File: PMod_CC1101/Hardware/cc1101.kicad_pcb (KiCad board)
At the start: 4 copper layers, 40.5 x 17 mm, 18 parts, among them J1 Conn_Coaxial, J2 Conn_02x06_Odd_Even, U1 CC1101RGPR

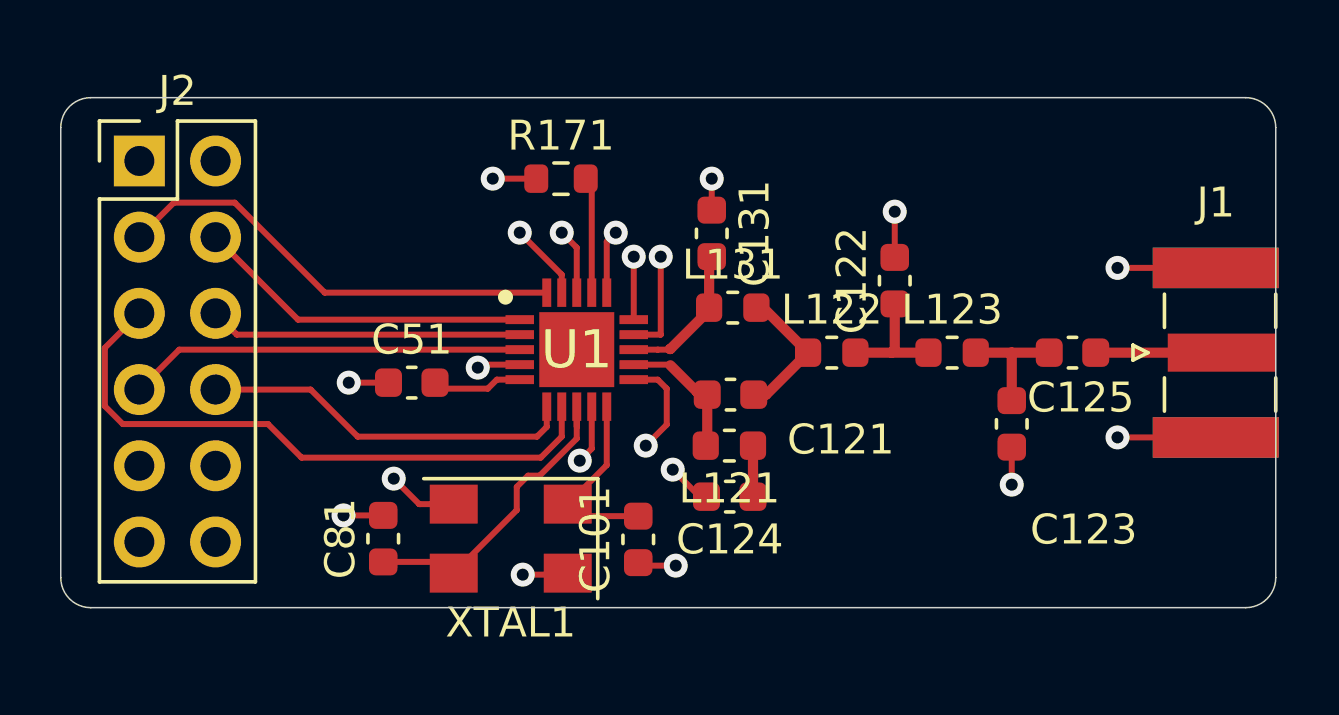
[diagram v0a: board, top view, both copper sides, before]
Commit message: Add GND filled zones
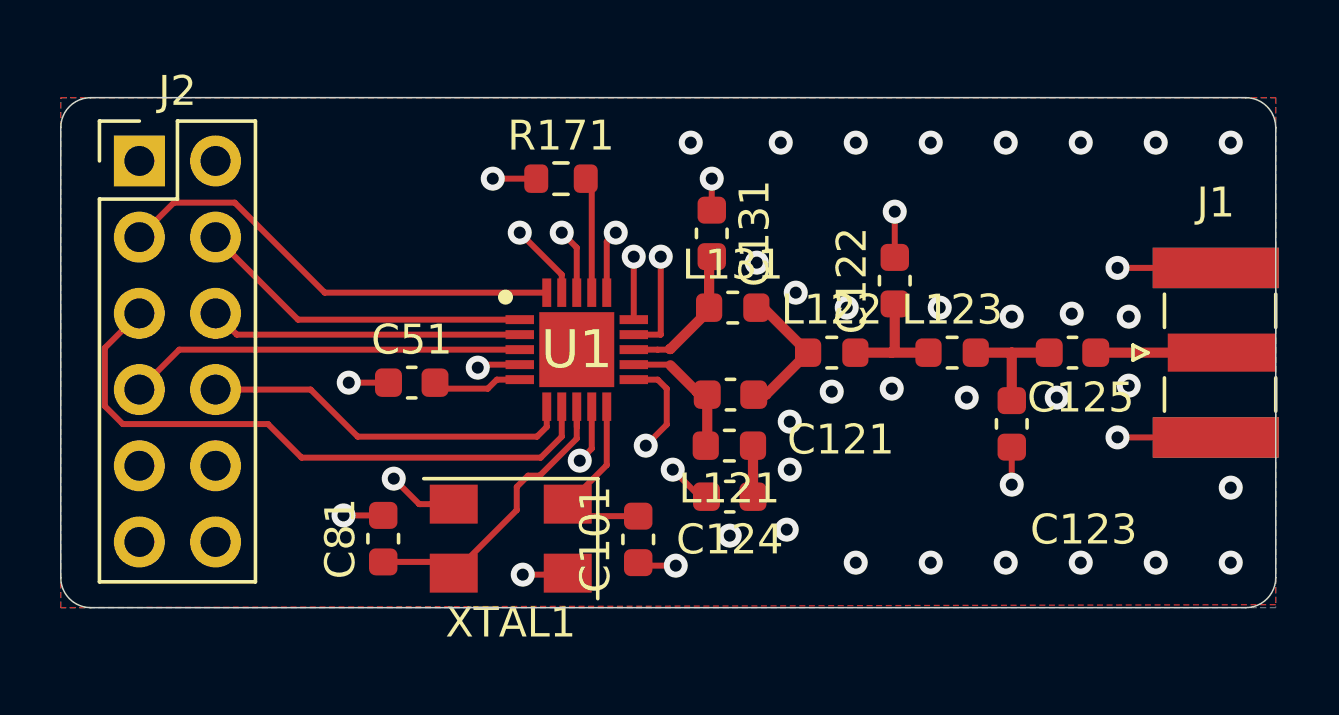
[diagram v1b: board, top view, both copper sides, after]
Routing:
- net GND: vias 14 -> 45
- added copper zone on B.Cu, net GND
- added copper zone on F.Cu, net GND
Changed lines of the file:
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@@
     (thickness 1.6)
     (drawings 10)
-    (tracks 139)
+    (tracks 170)
     (zones 0)
     (modules 18)
@@
     (1 In1.Cu signal hide)
     (2 In2.Cu signal hide)
-    (31 B.Cu signal)
+    (31 B.Cu signal hide)
     (32 B.Adhes user)
     (33 F.Adhes user)
@@
   (segment (start 142.95 68.05) (end 142.1 67.2) (width 0.2) (layer F.Cu) (net 2))
   (segment (start 144.1 68.05) (end 142.95 68.05) (width 0.2) (layer F.Cu) (net 2))
+  (via (at 158.7 64.2) (size 0.8) (drill 0.4) (layers F.Cu B.Cu) (net 2))
+  (via (at 157.2 61.5) (size 0.8) (drill 0.4) (layers F.Cu B.Cu) (net 2))
+  (via (at 160.3 61.5) (size 0.8) (drill 0.4) (layers F.Cu B.Cu) (net 2))
+  (via (at 162.7 61.8) (size 0.8) (drill 0.4) (layers F.Cu B.Cu) (net 2))
+  (via (at 161.2 64.5) (size 0.8) (drill 0.4) (layers F.Cu B.Cu) (net 2))
+  (via (at 164.2 64.5) (size 0.8) (drill 0.4) (layers F.Cu B.Cu) (net 2))
+  (via (at 166.6 64.1) (size 0.8) (drill 0.4) (layers F.Cu B.Cu) (net 2))
+  (via (at 166.6 61.8) (size 0.8) (drill 0.4) (layers F.Cu B.Cu) (net 2))
+  (via (at 164.7 61.7) (size 0.8) (drill 0.4) (layers F.Cu B.Cu) (net 2))
+  (via (at 156.7 64.3) (size 0.8) (drill 0.4) (layers F.Cu B.Cu) (net 2))
+  (via (at 154.2 60) (size 0.8) (drill 0.4) (layers F.Cu B.Cu) (net 2))
+  (via (at 155.3 65.3) (size 0.8) (drill 0.4) (layers F.Cu B.Cu) (net 2))
+  (via (at 155.3 66.9) (size 0.8) (drill 0.4) (layers F.Cu B.Cu) (net 2))
+  (via (at 155.2 68.9) (size 0.8) (drill 0.4) (layers F.Cu B.Cu) (net 2))
+  (via (at 153.3 69.1) (size 0.8) (drill 0.4) (layers F.Cu B.Cu) (net 2))
+  (via (at 155.5 61) (size 0.8) (drill 0.4) (layers F.Cu B.Cu) (net 2))
+  (via (at 170 70) (size 0.8) (drill 0.4) (layers F.Cu B.Cu) (net 2))
+  (via (at 167.5 70) (size 0.8) (drill 0.4) (layers F.Cu B.Cu) (net 2))
+  (via (at 165 70) (size 0.8) (drill 0.4) (layers F.Cu B.Cu) (net 2))
+  (via (at 162.5 70) (size 0.8) (drill 0.4) (layers F.Cu B.Cu) (net 2))
+  (via (at 160 70) (size 0.8) (drill 0.4) (layers F.Cu B.Cu) (net 2))
+  (via (at 157.5 70) (size 0.8) (drill 0.4) (layers F.Cu B.Cu) (net 2))
+  (via (at 170 67.5) (size 0.8) (drill 0.4) (layers F.Cu B.Cu) (net 2))
+  (via (at 170 56) (size 0.8) (drill 0.4) (layers F.Cu B.Cu) (net 2))
+  (via (at 167.5 56) (size 0.8) (drill 0.4) (layers F.Cu B.Cu) (net 2))
+  (via (at 165 56) (size 0.8) (drill 0.4) (layers F.Cu B.Cu) (net 2))
+  (via (at 162.5 56) (size 0.8) (drill 0.4) (layers F.Cu B.Cu) (net 2))
+  (via (at 160 56) (size 0.8) (drill 0.4) (layers F.Cu B.Cu) (net 2))
+  (via (at 155 56) (size 0.8) (drill 0.4) (layers F.Cu B.Cu) (net 2))
+  (via (at 157.5 56) (size 0.8) (drill 0.4) (layers F.Cu B.Cu) (net 2))
+  (via (at 152 56) (size 0.8) (drill 0.4) (layers F.Cu B.Cu) (net 2))
   (segment (start 148.2 64.8) (end 148.2 65.475) (width 0.2) (layer F.Cu) (net 3))
   (segment (start 146.2 68.25) (end 144.1 70.35) (width 0.2) (layer F.Cu) (net 3))
@@
     (connect_pads (clearance 0.508))
     (min_thickness 0.254)
+    (fill yes (arc_segments 32) (thermal_gap 0.508) (thermal_bridge_width 0.508))
+    (polygon
+      (pts
+        (xy 171.5 71.5) (xy 131 71.5) (xy 131 54.5) (xy 171.5 54.5)
+      )
+    )
+  )
+  (zone (net 2) (net_name GND) (layer F.Cu) (hatch edge 0.508)
+    (connect_pads (clearance 0.508))
+    (min_thickness 0.254)
+    (fill yes (arc_segments 32) (thermal_gap 0.508) (thermal_bridge_width 0.508))
+    (polygon
+      (pts
+        (xy 171.5 71.4) (xy 131 71.5) (xy 131 54.5) (xy 171.5 54.5)
+      )
+    )
+  )
+  (zone (net 2) (net_name GND) (layer B.Cu) (hatch edge 0.508)
+    (connect_pads (clearance 0.508))
+    (min_thickness 0.254)

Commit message: change the clearance for drc rules of cc1101 part
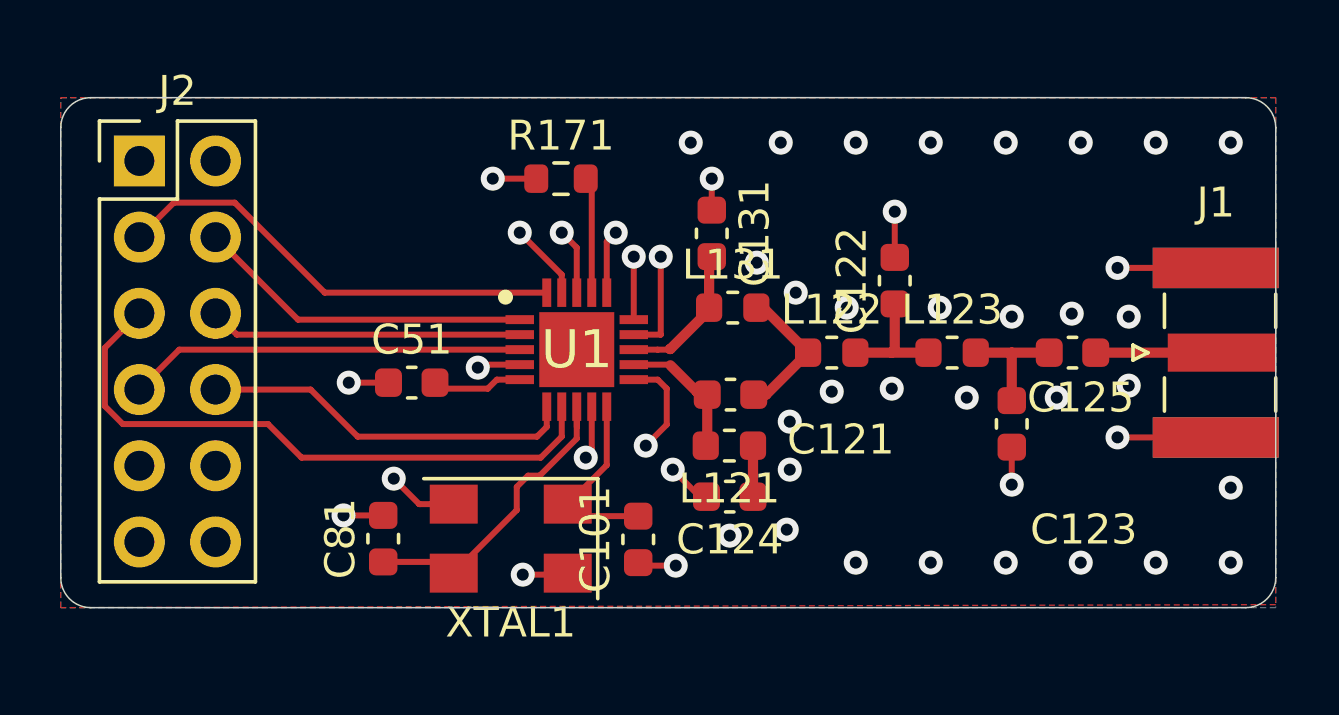
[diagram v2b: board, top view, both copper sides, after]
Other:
- net class Default: clearance 0.2 -> 0.1
- rule trace_clearance: 0.2 -> 0.1
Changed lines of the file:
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@@
     (thickness 1.6)
     (drawings 10)
-    (tracks 170)
+    (tracks 171)
     (zones 0)
     (modules 18)
@@
     (1 In1.Cu signal hide)
     (2 In2.Cu signal hide)
-    (31 B.Cu signal hide)
+    (31 B.Cu signal)
     (32 B.Adhes user)
     (33 F.Adhes user)
@@
     (user_trace_width 0.25)
     (user_trace_width 0.34036)
-    (trace_clearance 0.2)
+    (trace_clearance 0.1)
     (zone_clearance 0.508)
     (zone_45_only no)
@@
   (net 21 "Net-(R171-Pad2)")
   (net_class Default "This is the default net class."
-    (clearance 0.2)
+    (clearance 0.1)
     (trace_width 0.25)
     (via_dia 0.8)
@@
   (via (at 142.1 67.2) (size 0.8) (drill 0.4) (layers F.Cu B.Cu) (net 2))
   (via (at 144.9 63.5) (size 0.8) (drill 0.4) (layers F.Cu B.Cu) (net 11))
-  (via (at 148.3 66.6) (size 0.8) (drill 0.4) (layers F.Cu B.Cu) (net 11))
+  (via (at 148.5 66.5) (size 0.8) (drill 0.4) (layers F.Cu B.Cu) (net 11))
   (via (at 151.5 70.1) (size 0.8) (drill 0.4) (layers F.Cu B.Cu) (net 2))
   (via (at 146.4 70.4) (size 0.8) (drill 0.4) (layers F.Cu B.Cu) (net 2))
@@
   (via (at 150.1 59.8) (size 0.8) (drill 0.4) (layers F.Cu B.Cu) (net 11))
   (segment (start 148.7 66.2) (end 148.7 64.8) (width 0.2) (layer F.Cu) (net 11))
-  (segment (start 148.3 66.6) (end 148.7 66.2) (width 0.2) (layer F.Cu) (net 11))
   (segment (start 150.1 63.9) (end 150.9 63.9) (width 0.2) (layer F.Cu) (net 11))
   (segment (start 150.9 63.9) (end 151.2 64.2) (width 0.2) (layer F.Cu) (net 11))
@@
   (segment (start 145 63.4) (end 144.9 63.5) (width 0.2) (layer F.Cu) (net 11))
   (segment (start 146.3 63.4) (end 145 63.4) (width 0.2) (layer F.Cu) (net 11))
+  (segment (start 148.5 66.5) (end 148.7 66.3) (width 0.2) (layer F.Cu) (net 11))
+  (segment (start 148.7 66.3) (end 148.7 66.2) (width 0.2) (layer F.Cu) (net 11))
   (segment (start 140.9 65.8) (end 139.33 64.23) (width 0.2) (layer F.Cu) (net 12))
   (segment (start 146.875 65.8) (end 140.9 65.8) (width 0.2) (layer F.Cu) (net 12))
